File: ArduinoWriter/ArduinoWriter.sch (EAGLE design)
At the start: 27 parts, among them IC1 ATMEGA328-PU, IC2 TC74HC08AP, IC3 TC74HC32AP, Q1 HUSG-16.000-20, U1 ARRDUINOUNO-NOSILK

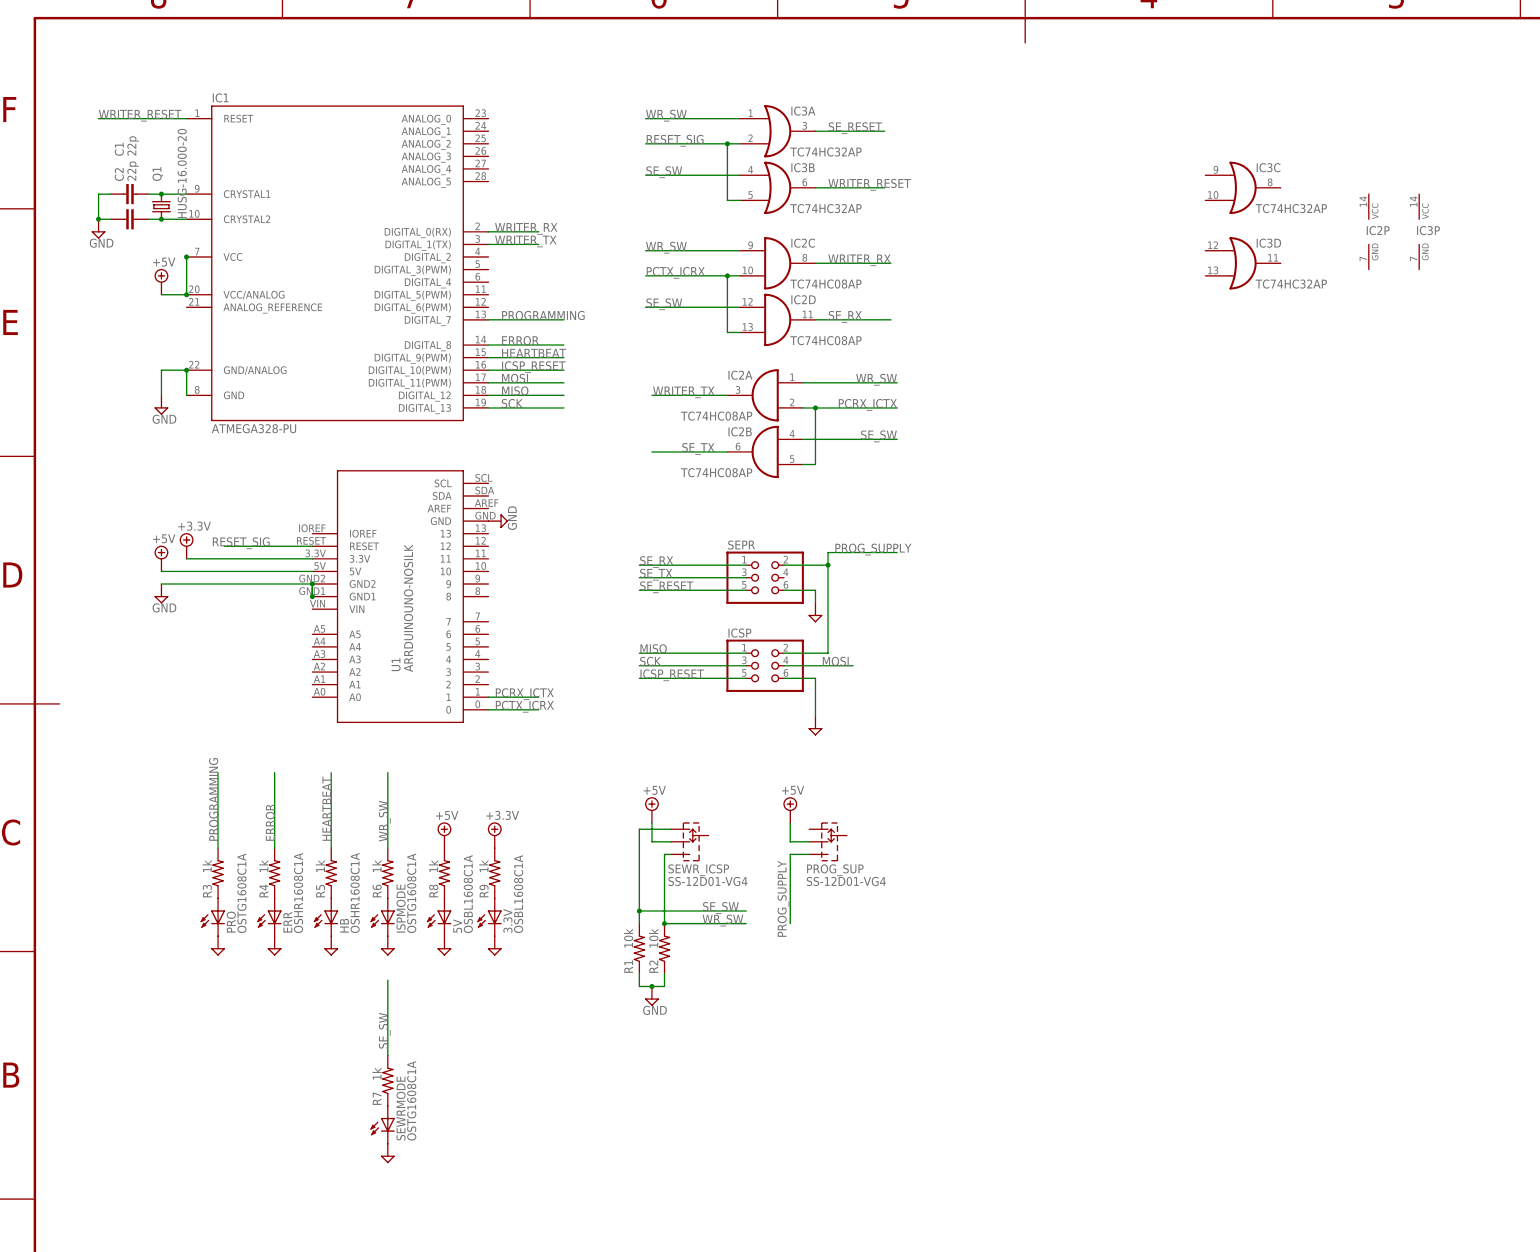
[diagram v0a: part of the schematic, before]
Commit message: レイアウト完了
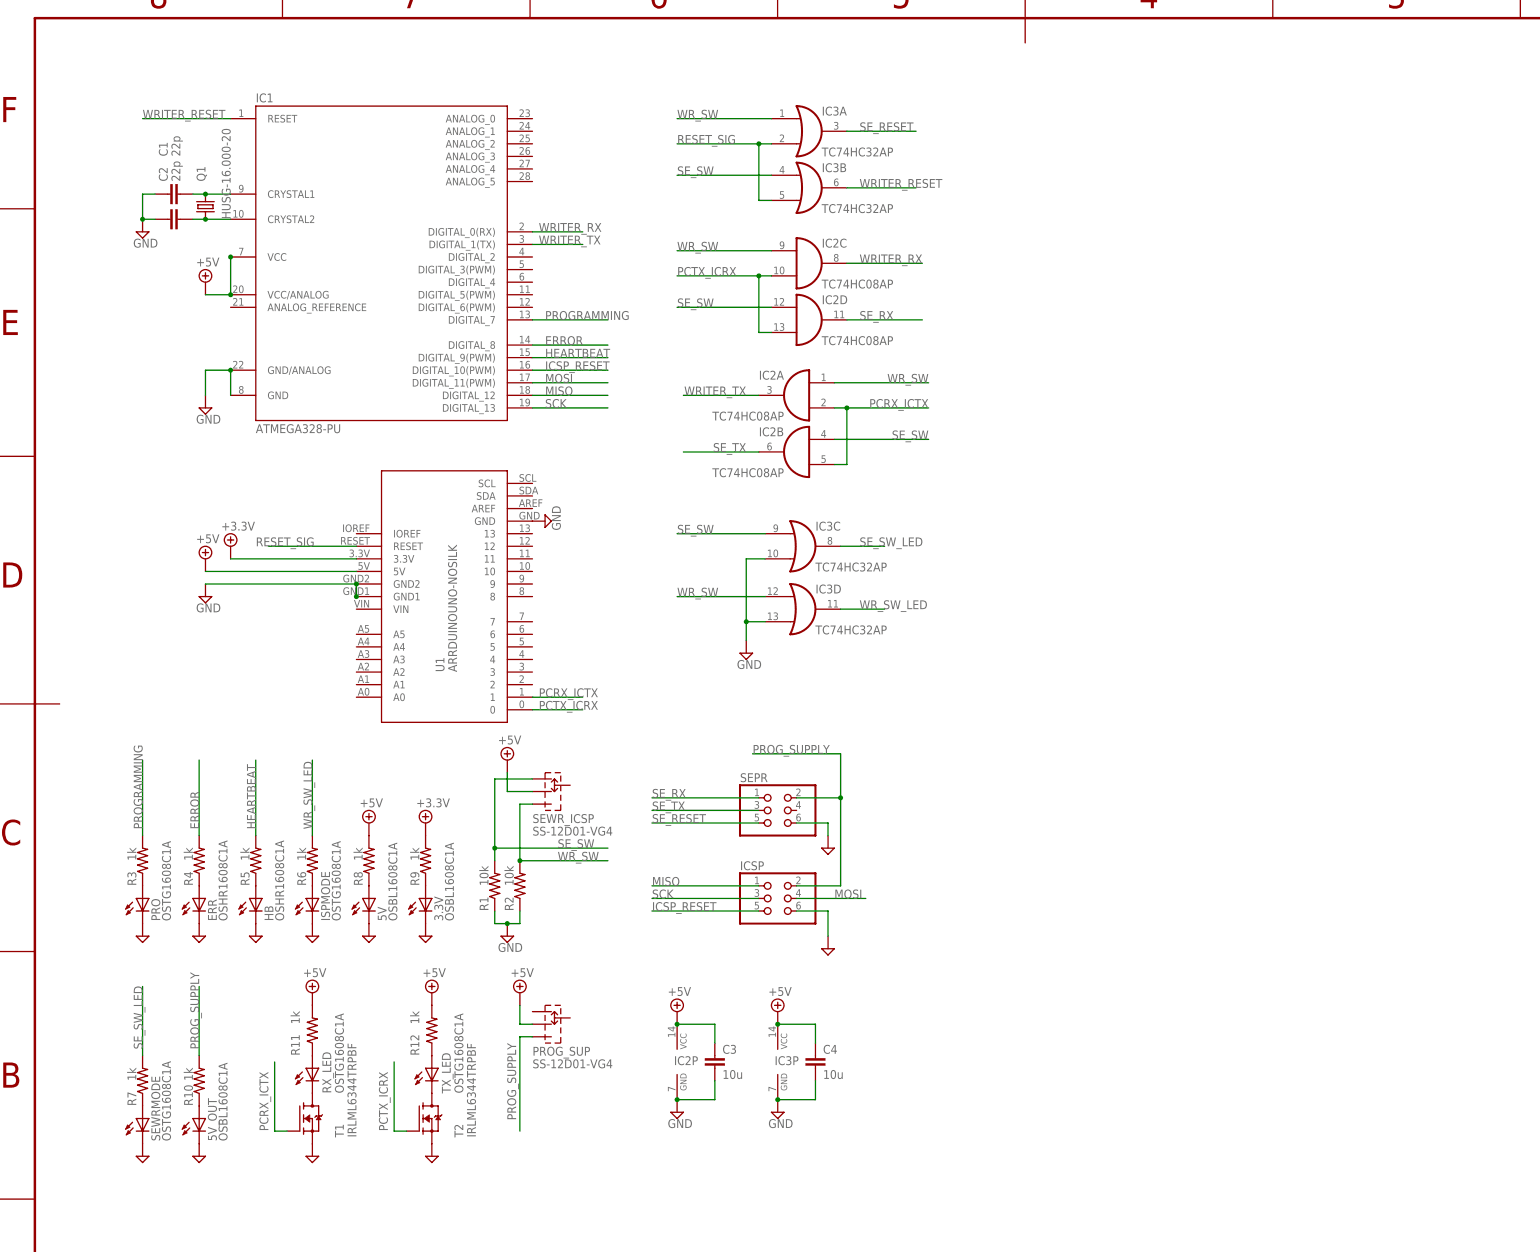
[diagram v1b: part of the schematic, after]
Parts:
- added 5V_OUT: OSBL1608C1A, LED:OSBL1608C1A
- added C3, C4: 10u, RCL:C2012
- added R10, R11, R12: 1k, RCL:R1608
- added RX_LED, TX_LED: OSTG1608C1A, LED:OSTG1608C1A
- added T1, T2: IRLML6344TRPBF, FET:IRLML6344TRPBF
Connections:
- new net N$10: 5V_OUT.A, R10.1
- new net N$11: RX_LED.C, T1.D
- new net N$12: T2.D, TX_LED.C
- new net N$13: R11.1, RX_LED.A
- new net N$14: R12.1, TX_LED.A
- new net SE_SW_LED: IC3C.O, R7.2
- new net WR_SW_LED: IC3D.O, R6.2
- net +5V: now also C3.1, C4.1, IC2P.VCC, IC3P.VCC, R11.2, R12.2
- net GND: now also 5V_OUT.C, C3.2, C4.2, IC2P.GND, IC3C.I1, IC3D.I1, IC3P.GND, T1.S, T2.S
- net PCRX_ICTX: now also T1.G
- net PCTX_ICRX: now also T2.G
- net PROG_SUPPLY: now also R10.2
- net SE_SW: now also IC3C.I0; no longer R7.2
- net WR_SW: now also IC3D.I0; no longer R6.2
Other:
- moved on the sheet: 3.3V, 5V, C1, C2, ERR, HB, IC1, IC2A, IC2B, IC2C, IC2D, IC2P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
